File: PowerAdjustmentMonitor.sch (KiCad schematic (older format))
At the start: 15 parts, among them U10 7805, U11 7805, U8 LM317, U9 LM317

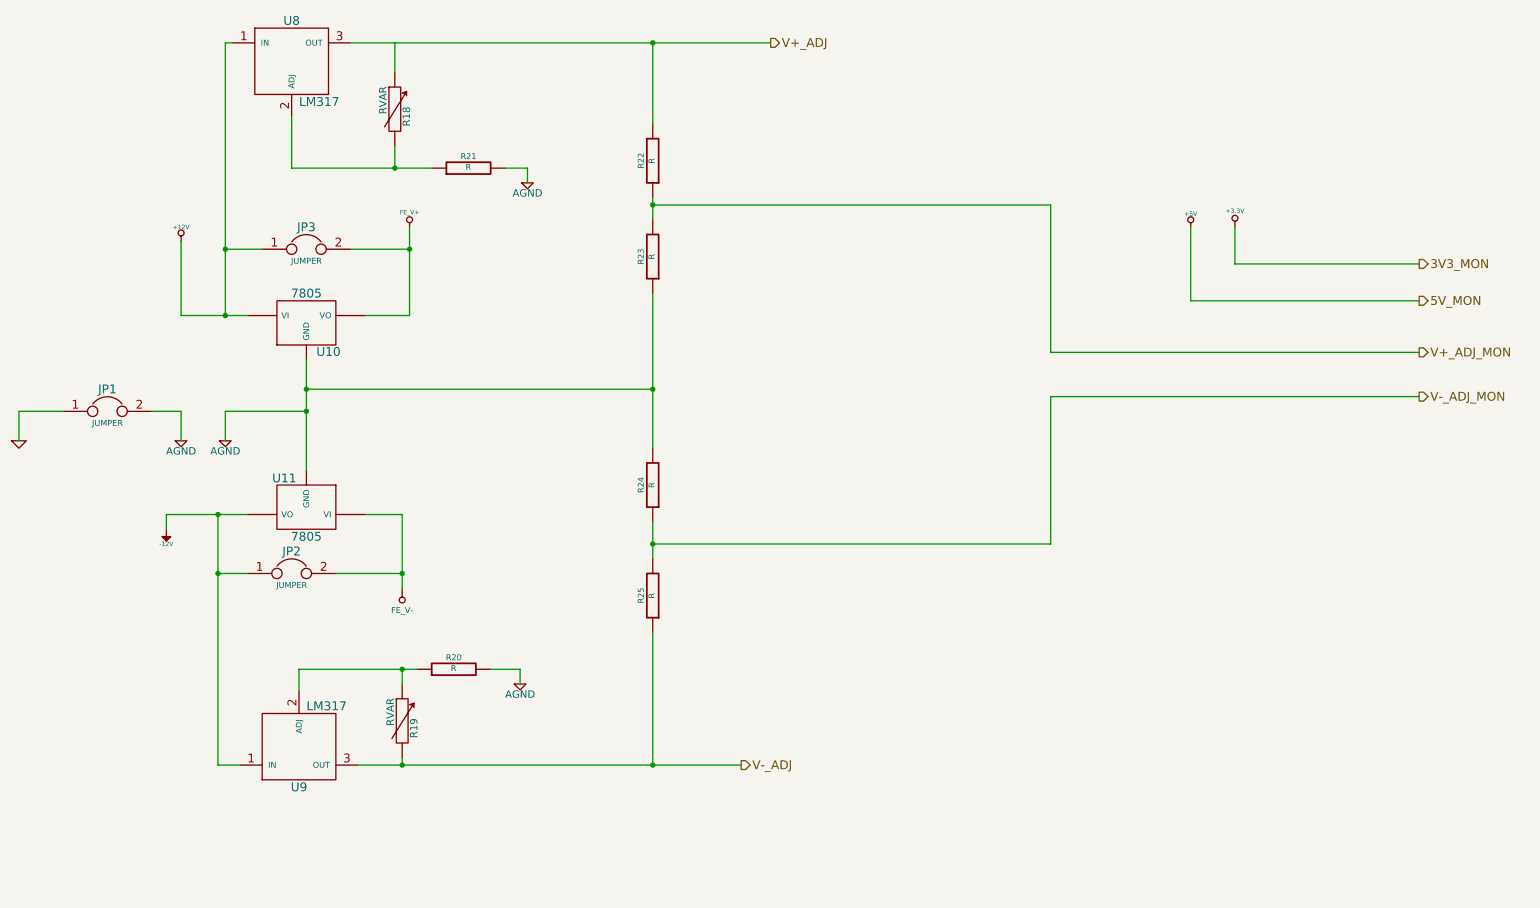
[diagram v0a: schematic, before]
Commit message: Power Adjustment: assc/placement
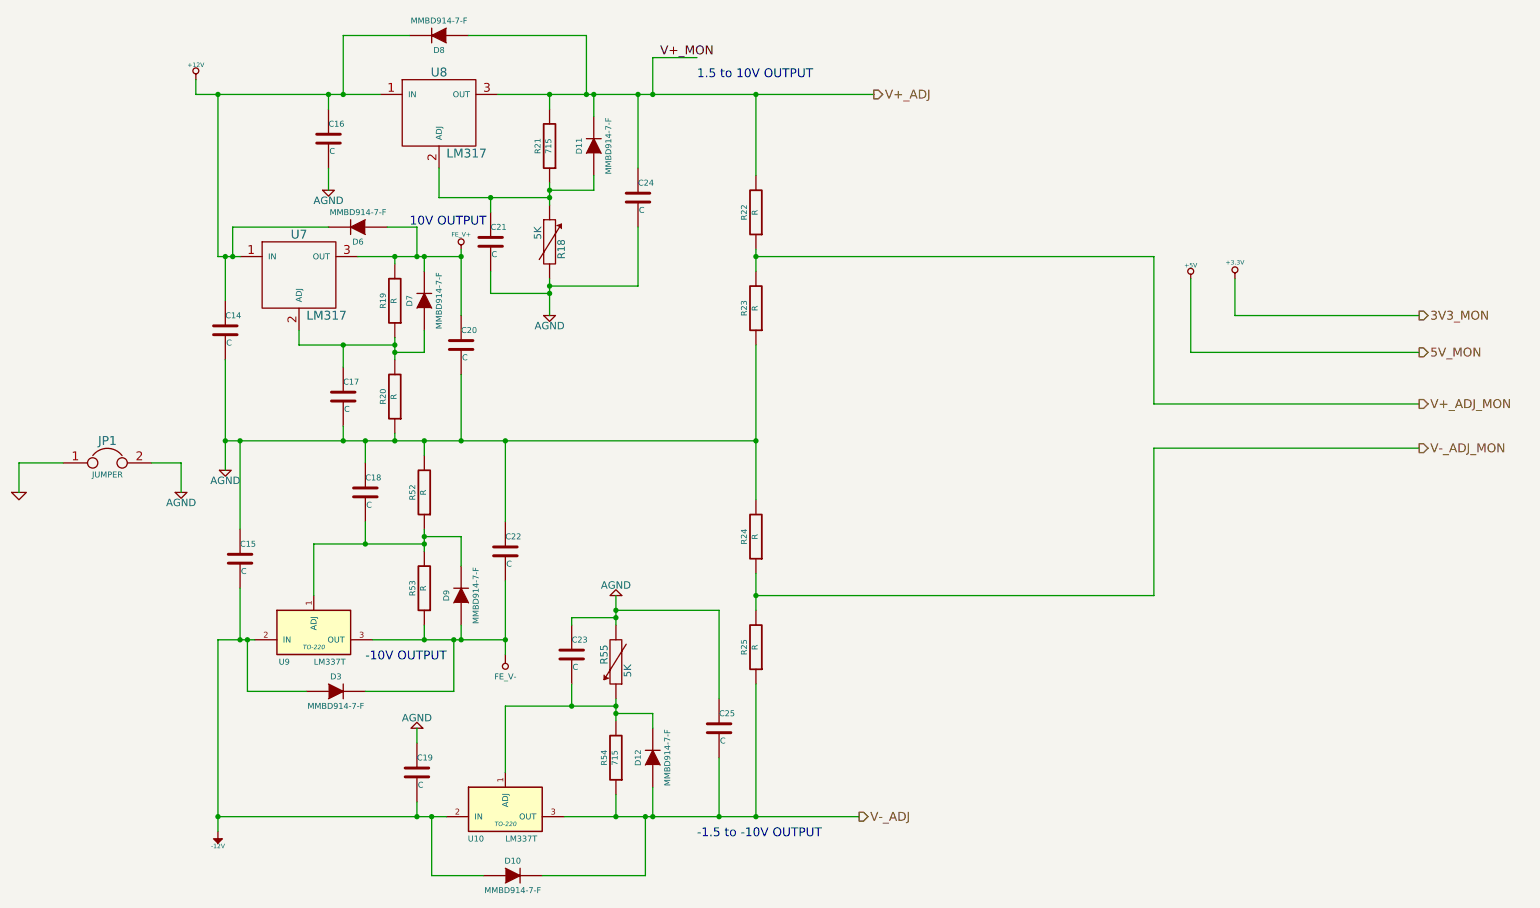
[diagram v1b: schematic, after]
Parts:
- removed JP2, JP3: JUMPER, ~, symbol JUMPER
- removed R19: RVAR, ~, symbol RVAR
- removed U10, U11: 7805, ~, symbol 7805
- removed U9: LM317, ~, symbol LM317
- added C14, C15, C16, C17, C18, C19, C20, C21, C22, C23, C24, C25: C, ~, symbol C
- added D10, D11, D12, D3, D6, D7, D8, D9: MMBD914-7-F, ~, symbol DIODE
- added R19, R52, R53: R, ~, symbol R
- added R54: 715, ~, symbol R
- added R55: 5K, ~, symbol RVAR
- added U10, U9: LM337T, TO-220, symbol LM337T
- added U7: LM317, ~, symbol LM317
- R18: value RVAR -> 5K
- R21: value R -> 715
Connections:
- net +12V: now also C14.1, C16.1, D6.2 (K), D8.2 (K), U7.1 (IN)
- net -12V: now also C15.2, C19.2, D10.1 (A), D3.1 (A), U10.2 (IN), U9.2 (IN)
- net AGND: now also R18.2, R20.1, C14.2, C15.1, C16.2, C17.2, C18.1, C19.1, C20.2, C21.2, C22.1, C23.1, C24.2, C25.1, R52.2, R55.2; no longer R20.2, R21.2
- net FE_V+: now also C20.1, D6.1 (A), D7.2 (K), R19.2, U7.3 (OUT)
- net FE_V-: now also C22.2, D3.2 (K), D9.1 (A), R53.1, U9.3 (OUT)
- net V+_ADJ: now also R21.2, C24.1, D11.2 (K), D8.1 (A)
- net V-_ADJ: now also C25.2, D10.2 (K), D12.1 (A), R54.1, U10.3 (OUT)
- net at R21.1, U8.2 (ADJ): now also R18.1, C21.1, D11.1 (A); no longer R18.2
- new net: C17.1, D7.1 (A), R19.1, R20.2, U7.2 (ADJ)
- new net: C18.2, D9.2 (K), R52.1, R53.2, U9.1 (ADJ)
- new net: C23.2, D12.2 (K), R54.2, R55.1, U10.1 (ADJ)
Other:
- note added: "-1.5 to -10V OUTPUT"
- note added: "-10V OUTPUT"
- note added: "1.5 to 10V OUTPUT"
- note added: "10V OUTPUT"
- moved on the sheet: JP1, R18, R21, R22, R23, R24, R25, U8
